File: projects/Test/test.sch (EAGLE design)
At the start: 47 parts, among them J2 1755529, U1 STM32F405RGT6, U2 CSD88584Q5DCT, U3 CSD88584Q5DCT, U4 CSD88584Q5DCT, Y1 ECS-80-S-4X

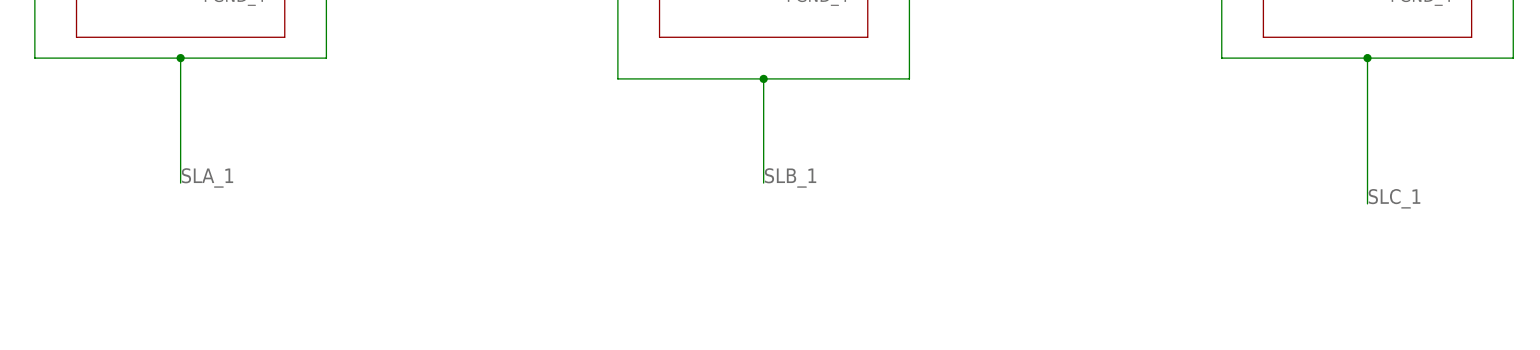
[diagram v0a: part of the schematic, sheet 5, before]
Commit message: some changes i made a while back and forgot to push
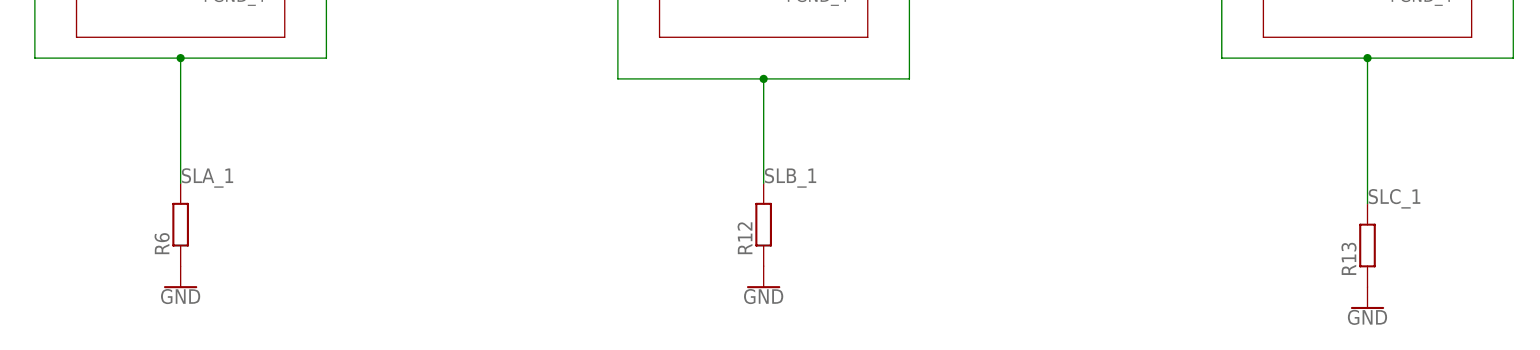
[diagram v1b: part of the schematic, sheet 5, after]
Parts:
- added R12, R13, R6: (no value), resistor-shunt:PMD
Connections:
- net GND: now also R12.2, R13.2, R6.2
- net SLA_1: now also R6.1
- net SLB_1: now also R12.1
- net SLC_1: now also R13.1
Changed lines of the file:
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@@
 <part name="U4" library="VESC_SHIT" library_urn="urn:adsk.eagle:library:11793053" deviceset="CSD88584Q5DCT" device=""/>
 <part name="U3" library="VESC_SHIT" library_urn="urn:adsk.eagle:library:11793053" deviceset="CSD88584Q5DCT" device=""/>
+<part name="R6" library="resistor-shunt" library_urn="urn:adsk.eagle:library:346" deviceset="PMD" device="" package3d_urn="urn:adsk.eagle:package:25216/1"/>
+<part name="R12" library="resistor-shunt" library_urn="urn:adsk.eagle:library:346" deviceset="PMD" device="" package3d_urn="urn:adsk.eagle:package:25216/1"/>
+<part name="R13" library="resistor-shunt" library_urn="urn:adsk.eagle:library:346" deviceset="PMD" device="" package3d_urn="urn:adsk.eagle:package:25216/1"/>
+<part name="GND12" library="SparkFun-PowerSymbols" library_urn="urn:adsk.eagle:library:530" deviceset="GND" device=""/>
+<part name="GND13" library="SparkFun-PowerSymbols" library_urn="urn:adsk.eagle:library:530" deviceset="GND" device=""/>
+<part name="GND14" library="SparkFun-PowerSymbols" library_urn="urn:adsk.eagle:library:530" deviceset="GND" device=""/>
 </parts>
 <sheets>
@@
 <attribute name="VALUE" x="50.5206" y="110.7186" size="2.0828" layer="96" ratio="6" rot="SR0"/>
 </instance>
+<instance part="R6" gate="G$1" x="55.88" y="43.18" smashed="yes" rot="R90">
+<attribute name="NAME" x="54.5084" y="39.37" size="1.778" layer="95" rot="R90"/>
+<attribute name="VALUE" x="58.801" y="39.37" size="1.778" layer="96" rot="R90"/>
+</instance>
+<instance part="R12" gate="G$1" x="127" y="43.18" smashed="yes" rot="R90">
+<attribute name="NAME" x="125.6284" y="39.37" size="1.778" layer="95" rot="R90"/>
+<attribute name="VALUE" x="129.921" y="39.37" size="1.778" layer="96" rot="R90"/>
+</instance>
+<instance part="R13" gate="G$1" x="200.66" y="40.64" smashed="yes" rot="R90">
+<attribute name="NAME" x="199.2884" y="36.83" size="1.778" layer="95" rot="R90"/>
+<attribute name="VALUE" x="203.581" y="36.83" size="1.778" layer="96" rot="R90"/>
+</instance>
+<instance part="GND12" gate="1" x="55.88" y="35.56" smashed="yes">
+<attribute name="VALUE" x="55.88" y="35.306" size="1.778" layer="96" align="top-center"/>
+</instance>
+<instance part="GND13" gate="1" x="127" y="35.56" smashed="yes">
+<attribute name="VALUE" x="127" y="35.306" size="1.778" layer="96" align="top-center"/>
+</instance>
+<instance part="GND14" gate="1" x="200.66" y="33.02" smashed="yes">
+<attribute name="VALUE" x="200.66" y="32.766" size="1.778" layer="96" align="top-center"/>
+</instance>
 </instances>
 <busses>
@@
 <junction x="73.66" y="83.82"/>
 <pinref part="U3" gate="A" pin="PGND"/>
+<pinref part="R6" gate="G$1" pin="1"/>
 </segment>
 </net>
@@
 <junction x="144.78" y="83.82"/>
 <pinref part="U4" gate="A" pin="PGND"/>
+<pinref part="R12" gate="G$1" pin="1"/>
 </segment>
 </net>
@@
 <junction x="218.44" y="83.82"/>
 <pinref part="U2" gate="A" pin="PGND"/>
+<pinref part="R13" gate="G$1" pin="1"/>
 </segment>
 </net>
@@
 </segment>
 </net>
+<net name="GND" class="0">
+<segment>
+<pinref part="GND12" gate="1" pin="GND"/>
+<pinref part="R6" gate="G$1" pin="2"/>
+</segment>
+<segment>
+<pinref part="GND13" gate="1" pin="GND"/>
+<pinref part="R12" gate="G$1" pin="2"/>
+</segment>
+<segment>
+<pinref part="GND14" gate="1" pin="GND"/>
+<pinref part="R13" gate="G$1" pin="2"/>
+</segment>
+</net>
